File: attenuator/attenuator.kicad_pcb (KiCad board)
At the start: 2 copper layers, 127.6 x 33.1 mm, 65 parts, among them J1 Conn_Coaxial, J11 Conn_02x07_Odd_Even, J2 Conn_Coaxial, U1 4259-63, U10 4259-63, U2 4259-63, U3 4259-63, U4 4259-63, U5 4259-63, U6 4259-63, U7 4259-63, U8 4259-63, U9 4259-63

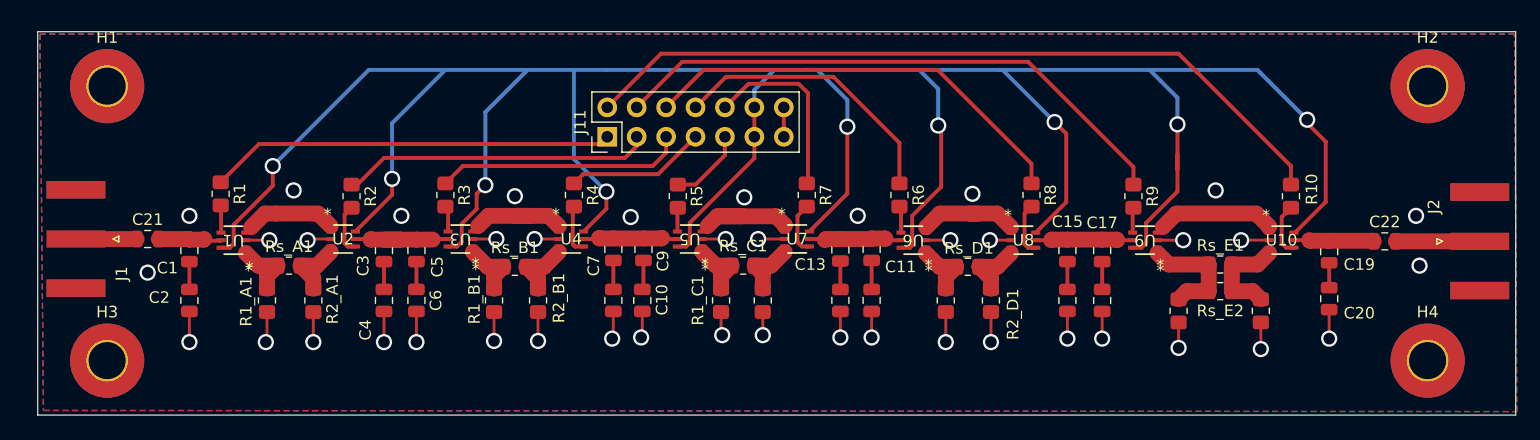
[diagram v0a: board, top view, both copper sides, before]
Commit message: pcb improve it
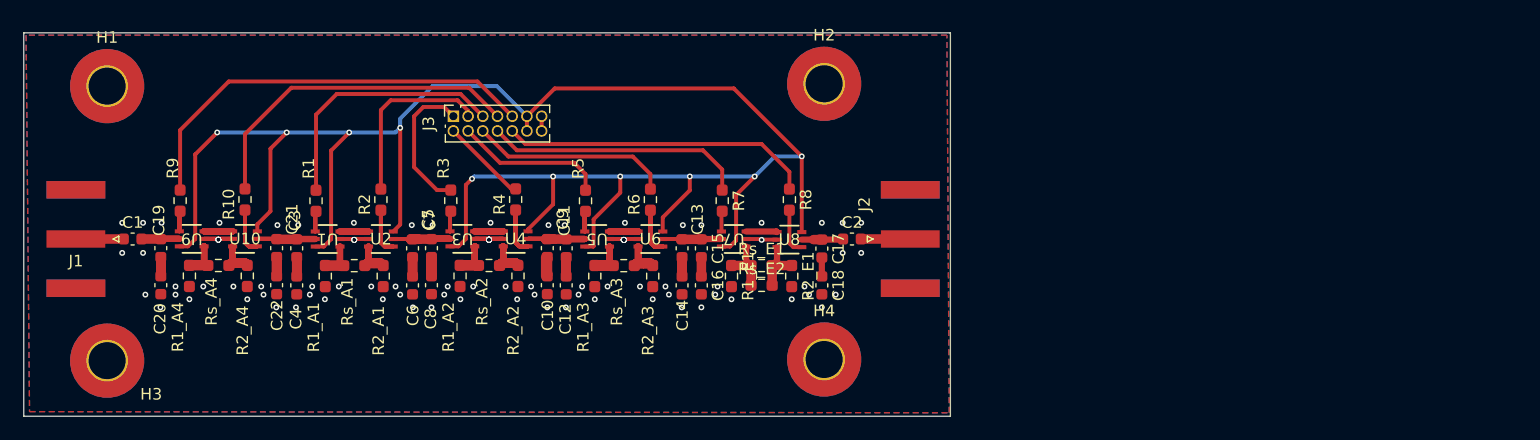
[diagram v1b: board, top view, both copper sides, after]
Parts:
- removed J11: Conn_02x07_Odd_Even, Connector_PinHeader_2.54mm:PinHeader_2x07_P2.54mm_Vertical
- removed R1_B1, R2_B1: 115, Resistor_SMD:R_0805_2012Metric_Pad1.20x1.40mm_HandSolder
- removed R1_C1, R2_C1: 221, Resistor_SMD:R_0805_2012Metric_Pad1.20x1.40mm_HandSolder
- removed R1_D1, R2_D1: 432, Resistor_SMD:R_0805_2012Metric_Pad1.20x1.40mm_HandSolder
- removed Rs_B1: 52.3, Resistor_SMD:R_0805_2012Metric_Pad1.20x1.40mm_HandSolder
- removed Rs_C1: 23.7, Resistor_SMD:R_0805_2012Metric_Pad1.20x1.40mm_HandSolder
- removed Rs_D1: 11.5, Resistor_SMD:R_0805_2012Metric_Pad1.20x1.40mm_HandSolder
- added J3: Conn_02x07_Odd_Even, Connector_PinSocket_1.27mm:PinSocket_2x07_P1.27mm_Vertical, F.Cu at (68.0, 33.2)
- added R1_A2: 221, Resistor_SMD:R_0603_1608Metric_Pad0.98x0.95mm_HandSolder, F.Cu at (68.6, 47.0)
- added R1_A3: 432, Resistor_SMD:R_0603_1608Metric_Pad0.98x0.95mm_HandSolder, F.Cu at (80.2, 47.0)
- added R1_A4: 68.1, Resistor_SMD:R_0603_1608Metric_Pad0.98x0.95mm_HandSolder, F.Cu at (45.2, 47.0)
- added R2_A2: 221, Resistor_SMD:R_0603_1608Metric_Pad0.98x0.95mm_HandSolder, F.Cu at (73.6, 47.0)
- added R2_A3: 432, Resistor_SMD:R_0603_1608Metric_Pad0.98x0.95mm_HandSolder, F.Cu at (85.2, 47.0)
- added R2_A4: 68.1, Resistor_SMD:R_0603_1608Metric_Pad0.98x0.95mm_HandSolder, F.Cu at (50.2, 47.0)
- added Rs_A2: 23.7, Resistor_SMD:R_0603_1608Metric_Pad0.98x0.95mm_HandSolder, F.Cu at (71.1, 46.1)
- added Rs_A3: 11.5, Resistor_SMD:R_0603_1608Metric_Pad0.98x0.95mm_HandSolder, F.Cu at (82.7, 46.1)
- added Rs_A4: 154, Resistor_SMD:R_0603_1608Metric_Pad0.98x0.95mm_HandSolder, F.Cu at (47.7, 46.1)
- C1: value 0.5p -> 1P; footprint Capacitor_SMD:C_0805_2012Metric -> Capacitor_SMD:C_0603_1608Metric
- C10, C11, C12, C13, C14, C15, C16, C17, C18, C19, C20, C3, C4, C5, C6, C7, C8, C9: footprint Capacitor_SMD:C_0805_2012Metric -> Capacitor_SMD:C_0603_1608Metric
- C2: value 0.5p -> C; footprint Capacitor_SMD:C_0805_2012Metric -> Capacitor_SMD:C_0603_1608Metric
- C21: value 1P -> 0.5p; footprint Capacitor_SMD:C_0805_2012Metric -> Capacitor_SMD:C_0603_1608Metric
- C22: value C -> 0.5p; footprint Capacitor_SMD:C_0805_2012Metric -> Capacitor_SMD:C_0603_1608Metric
- R1, R10, R1_E1, R2, R2_E1, R3, R4, R5, R6, R7, R8, R9: footprint Resistor_SMD:R_0805_2012Metric_Pad1.20x1.40mm_HandSolder -> Resistor_SMD:R_0603_1608Metric_Pad0.98x0.95mm_HandSolder
- R1_A1, R2_A1: value 68.1 -> 115; footprint Resistor_SMD:R_0805_2012Metric_Pad1.20x1.40mm_HandSolder -> Resistor_SMD:R_0603_1608Metric_Pad0.98x0.95mm_HandSolder
- Rs_A1: value 154 -> 52.3; footprint Resistor_SMD:R_0805_2012Metric_Pad1.20x1.40mm_HandSolder -> Resistor_SMD:R_0603_1608Metric_Pad0.98x0.95mm_HandSolder
- Rs_E1, Rs_E2: value 11.5 -> 111.5; footprint Resistor_SMD:R_0805_2012Metric_Pad1.20x1.40mm_HandSolder -> Resistor_SMD:R_0603_1608Metric_Pad0.98x0.95mm_HandSolder
- moved C20 100.9 mm to (42.7, 47.8)
- moved C19 100.9 mm to (42.7, 44.6)
- moved C22 95.7 mm to (52.7, 47.8), turned to -90 degrees
- moved R10 90.3 mm to (50.0, 40.4)
- moved U10 89.5 mm to (50.0, 43.8)
- moved R9 82.3 mm to (44.4, 40.5)
- moved U9 82.3 mm to (45.4, 43.8)
- moved C2 57.4 mm to (102.4, 43.8), turned to 0 degrees
- moved H2 52.1 mm to (100.0, 30.4)
- moved H4 52.1 mm to (100.0, 54.2)
- moved J2 49.2 mm to (107.4, 43.8)
- moved R2_E1 40.6 mm to (97.2, 47.0)
- moved Rs_E2 39.6 mm to (94.6, 47.8)
- moved Rs_E1 39.6 mm to (94.6, 46.1)
- moved R1_E1 38.7 mm to (92.0, 47.0)
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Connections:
- net /switch/RF1 renamed Net-(U1-RF1)
- net /switch/RF2 renamed Net-(U1-RF2)
- net /switch1/RF2 renamed Net-(U2-RF2)
- net /switch2/RF2 renamed Net-(U3-RF2)
- net /switch8/RF2 renamed Net-(U10-RF1)
- C1 pad 1: /switch/RFC -> Net-(J1-In)
- C1 pad 2: Net-(C1-Pad2) -> /attenuator_block/RFC_IN
- C11 pad 1: /switch5/RFC -> /attenuator_block2/RFC_OUT
- C13 pad 1: /switch5/RFC -> /attenuator_block3/RFC_OUT
- C15 pad 1: /switch7/RFC -> /attenuator_block3/RFC_OUT
- C17 pad 1: /switch7/RFC -> /attenuator_block_v2/RFC_OUT
- C19 pad 1: /switch9/RFC -> /attenuator_block/RFC_IN
- C2 pad 1: Net-(C1-Pad2) -> /attenuator_block_v2/RFC_OUT
- C2 pad 2: GND -> Net-(J2-In)
- C21 pad 1: Net-(J1-In) -> /attenuator_block/RFC_OUT
- C21 pad 2: /switch/RFC -> Net-(C21-Pad2)
- C22 pad 1: /switch9/RFC -> Net-(C21-Pad2)
- C22 pad 2: Net-(J2-In) -> GND
- C3 pad 1: /switch1/RFC -> /attenuator_block/RFC_OUT
- C5 pad 1: /switch1/RFC -> /attenuator_block1/RFC_OUT
- C7 pad 1: /switch3/RFC -> /attenuator_block1/RFC_OUT
- C9 pad 1: /switch3/RFC -> /attenuator_block2/RFC_OUT
- R1 pad 1: /CTRL_1 -> /CTRL_3
- R10 pad 1: /CTRL_10 -> /CTRL_2
- R1_E1 pad 1: /switch8/RF1 -> Net-(U7-RF1)
- R2 pad 1: /CTRL_2 -> /CTRL_4
- R2_E1 pad 1: /switch9/RF2 -> Net-(U8-RF2)
- R3 pad 1: /CTRL_3 -> /CTRL_5
- R4 pad 1: /CTRL_4 -> /CTRL_6
- R5 pad 1: /CTRL_8 -> /CTRL_7
- R6 pad 1: /CTRL_6 -> /CTRL_8
- R7 pad 1: /CTRL_7 -> /CTRL_9
- R8 pad 1: /CTRL_5 -> /CTRL_10
- R9 pad 1: /CTRL_9 -> /CTRL_1
- Rs_E1 pad 1: /switch8/RF1 -> Net-(U7-RF1)
- Rs_E1 pad 2: /switch9/RF2 -> Net-(U8-RF2)
- Rs_E2 pad 1: /switch8/RF1 -> Net-(U7-RF1)
- Rs_E2 pad 2: /switch9/RF2 -> Net-(U8-RF2)
- U1 pad 5: /switch/RFC -> /attenuator_block/RFC_OUT
- U10 pad 3: /switch9/RF2 -> Net-(U10-RF2)
- U10 pad 5: /switch9/RFC -> /attenuator_block/RFC_OUT
- U2 pad 5: /switch1/RFC -> /attenuator_block1/RFC_OUT
- U3 pad 1: /switch2/RF1 -> Net-(U3-RF1)
- U3 pad 5: /switch1/RFC -> /attenuator_block1/RFC_OUT
- U4 pad 3: /switch4/RF2 -> Net-(U4-RF2)
- U4 pad 5: /switch3/RFC -> /attenuator_block2/RFC_OUT
- U5 pad 1: /switch3/RF1 -> Net-(U5-RF1)
- U5 pad 3: /switch3/RF2 -> Net-(U5-RF2)
- U5 pad 5: /switch3/RFC -> /attenuator_block2/RFC_OUT
- U6 pad 1: /switch6/RF1 -> Net-(U5-RF2)
- U6 pad 3: /switch6/RF2 -> Net-(U6-RF2)
- U6 pad 5: /switch5/RFC -> /attenuator_block3/RFC_OUT
- U7 pad 1: /switch3/RF2 -> Net-(U7-RF1)
- U7 pad 3: /switch5/RF2 -> Net-(U7-RF2)
- U7 pad 5: /switch5/RFC -> /attenuator_block3/RFC_OUT
- U8 pad 1: /switch6/RF2 -> Net-(U7-RF2)
- U8 pad 3: /switch7/RF2 -> Net-(U8-RF2)
- U8 pad 5: /switch7/RFC -> /attenuator_block_v2/RFC_OUT
- U9 pad 1: /switch8/RF1 -> Net-(U9-RF1)
- U9 pad 5: /switch7/RFC -> /attenuator_block/RFC_IN
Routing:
- net /3V: track 263.0 -> 169.9 mm, vias 9 -> 10
- net /CTRL_10: track 66.7 -> 26.9 mm
- net /CTRL_9: track 49.8 -> 22.6 mm
- net /CTRL_5: track 37.9 -> 12.4 mm
- net /attenuator_block2/RFC_OUT: track 0.00 -> 22.0 mm
- net Net-(U5-RF1): track 0.00 -> 22.0 mm
- net Net-(U3-RF1): track 0.00 -> 22.0 mm
- net Net-(U6-CTRL): track 2.31 -> 24.1 mm
- net Net-(U4-RF2): track 0.00 -> 21.2 mm
- net Net-(U6-RF2): track 0.00 -> 21.2 mm
- net GND: track 72.1 -> 52.0 mm, vias 42 -> 93
- net Net-(U4-CTRL): track 4.31 -> 24.1 mm
- net /switch6/RF2: track 18.5 -> 0.00 mm
- net /switch3/RF2: track 17.9 -> 0.00 mm
- net /attenuator_block1/RFC_OUT: track 0.00 -> 17.1 mm
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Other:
- board size 127.6 x 33.1 mm -> 80 x 33.1 mm
